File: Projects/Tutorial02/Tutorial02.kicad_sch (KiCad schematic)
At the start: 16 parts, among them J1 FTDI Programmer, J2 Arduino PIN0 - PIN7, J3 Arduino A0 - A5, J4 Power & Ground Terminal, J5 Versorgungsspannung, J6 Arduino PIN8 - PIN13, U1 ATMEGA328P-PU, Y1 Crystal

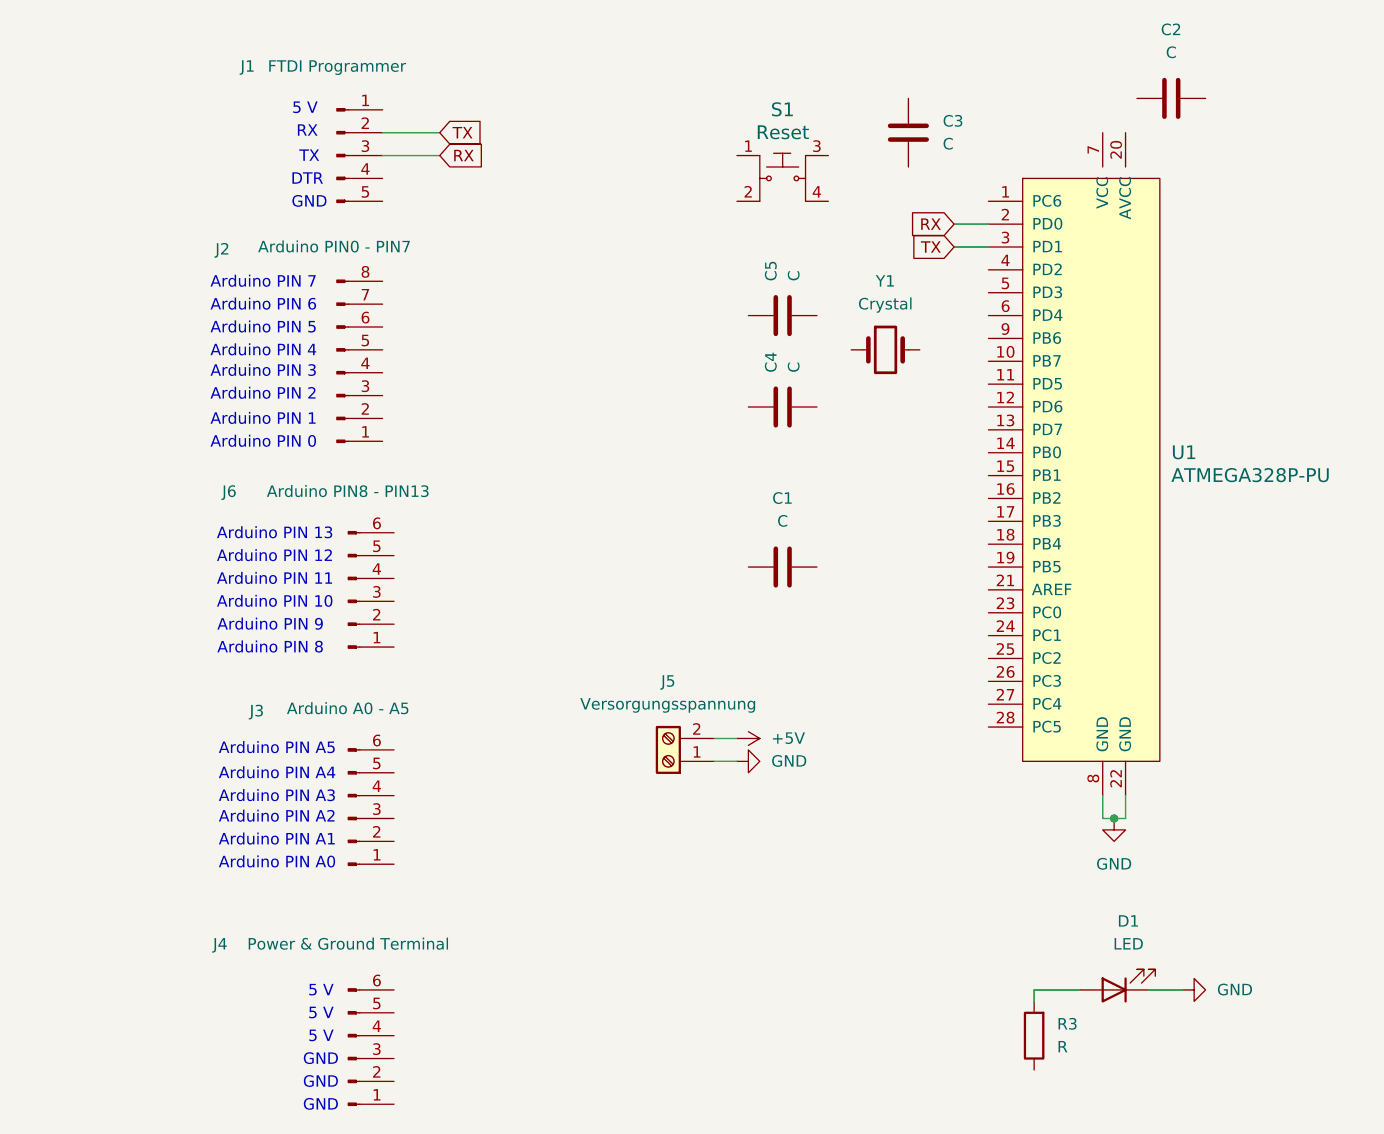
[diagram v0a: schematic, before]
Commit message: 20251209 tutorial02
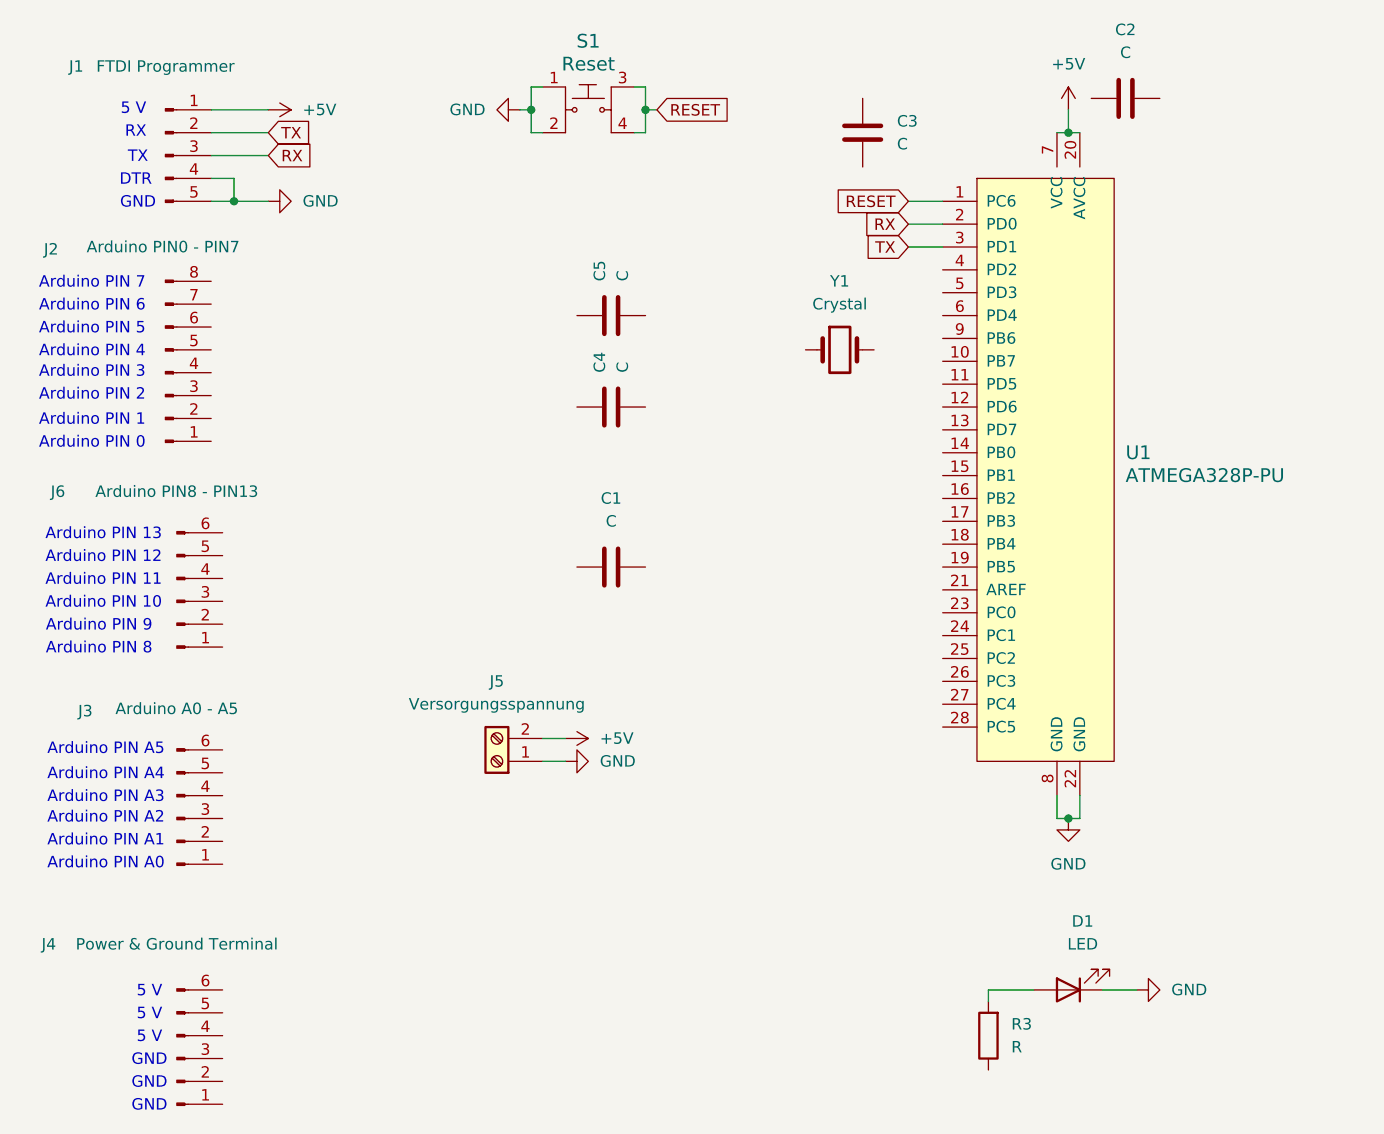
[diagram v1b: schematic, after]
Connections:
- net +5V: now also J1.1 (Pin_1), U1.20 (AVCC), U1.7 (VCC)
- net GND: now also J1.4 (Pin_4), J1.5 (Pin_5), S1.1, S1.2
- net RESET: now reaches S1.3
- net RESET: now also S1.4, U1.1 (PC6)
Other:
- moved on the sheet: C1, C2, C3, C4, C5, D1, J1, J2, J3, J4, J5, J6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
